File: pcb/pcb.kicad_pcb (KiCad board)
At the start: 2 copper layers, 165.5 x 101.1 mm, 59 parts, among them J1 N!N, J2 Conn_01x02_Socket, J4 Display_nice-view, J8 Conn_01x12_Socket, J9 Conn_01x12_Socket, SW1 Switch, SW10 Switch, SW11 Switch, SW12 Switch, SW13 Switch, SW14 Switch, SW15 Switch, SW16 Switch, SW17 Switch, SW18 Switch, SW19 Switch, SW2 Switch, SW20 Switch, SW21 SW_Push, SW22 SW_SPDT, SW3 Switch, SW4 Switch, SW5 Switch, SW6 Switch, SW7 Switch, SW8 Switch, SW9 Switch

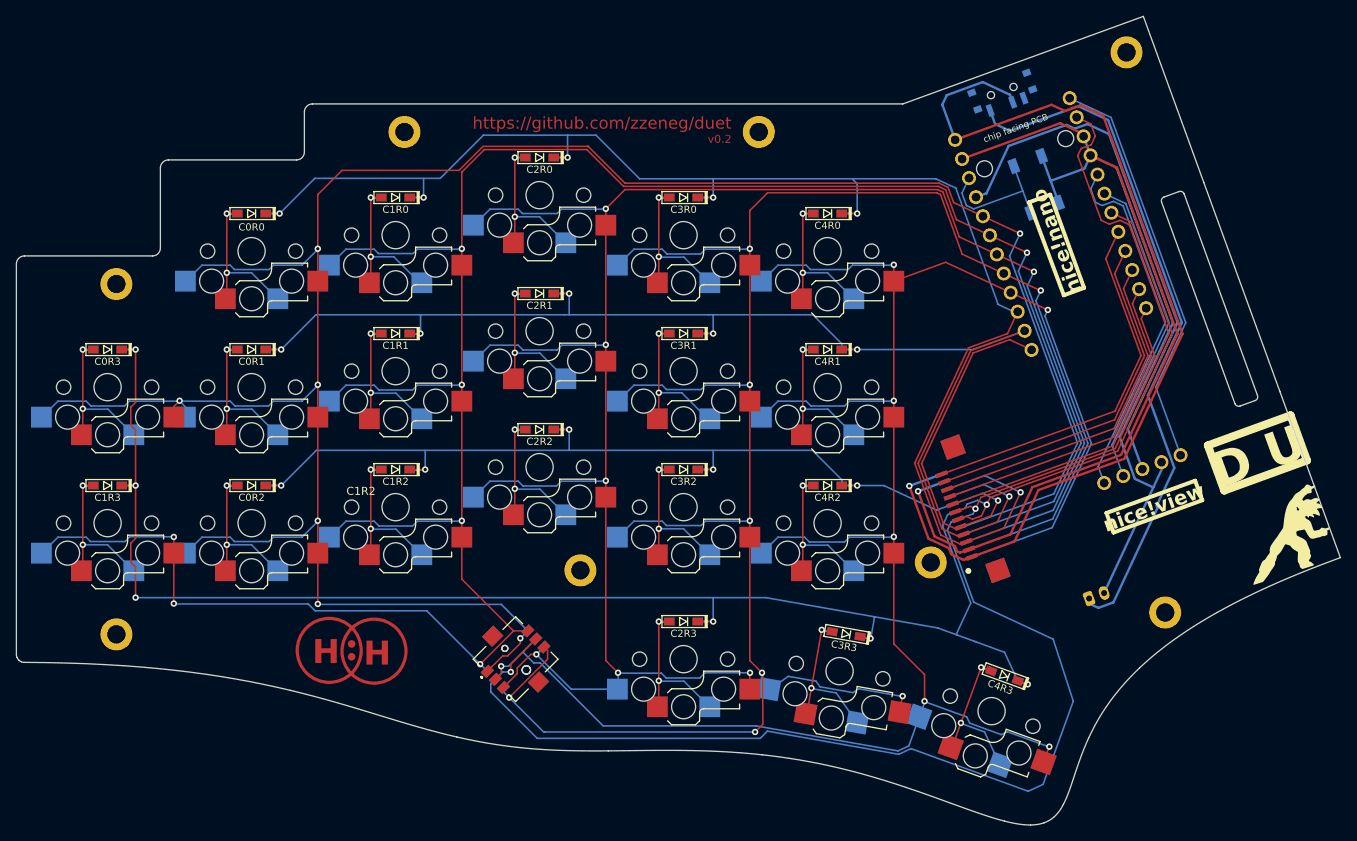
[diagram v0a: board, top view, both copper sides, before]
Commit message: small updates
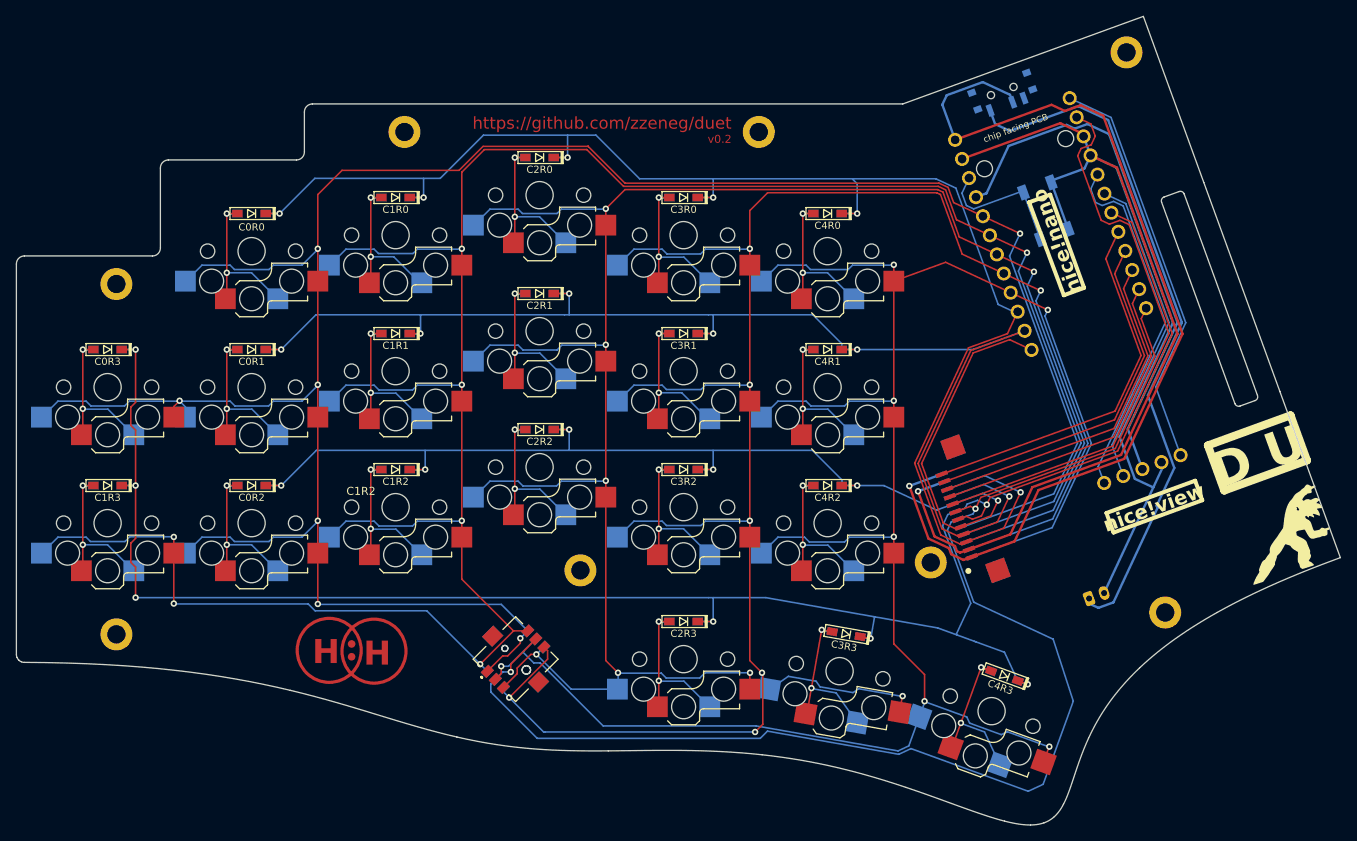
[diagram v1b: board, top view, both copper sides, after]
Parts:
- moved SW21 3.50 mm to (164.8, 53.9)
